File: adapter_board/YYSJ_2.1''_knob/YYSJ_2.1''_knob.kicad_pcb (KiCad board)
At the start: 2 copper layers, 80 x 80 mm, 12 parts, among them J1 USB_C_Receptacle_USB2.0, J2 FPC 10, J3 Conn_01x10

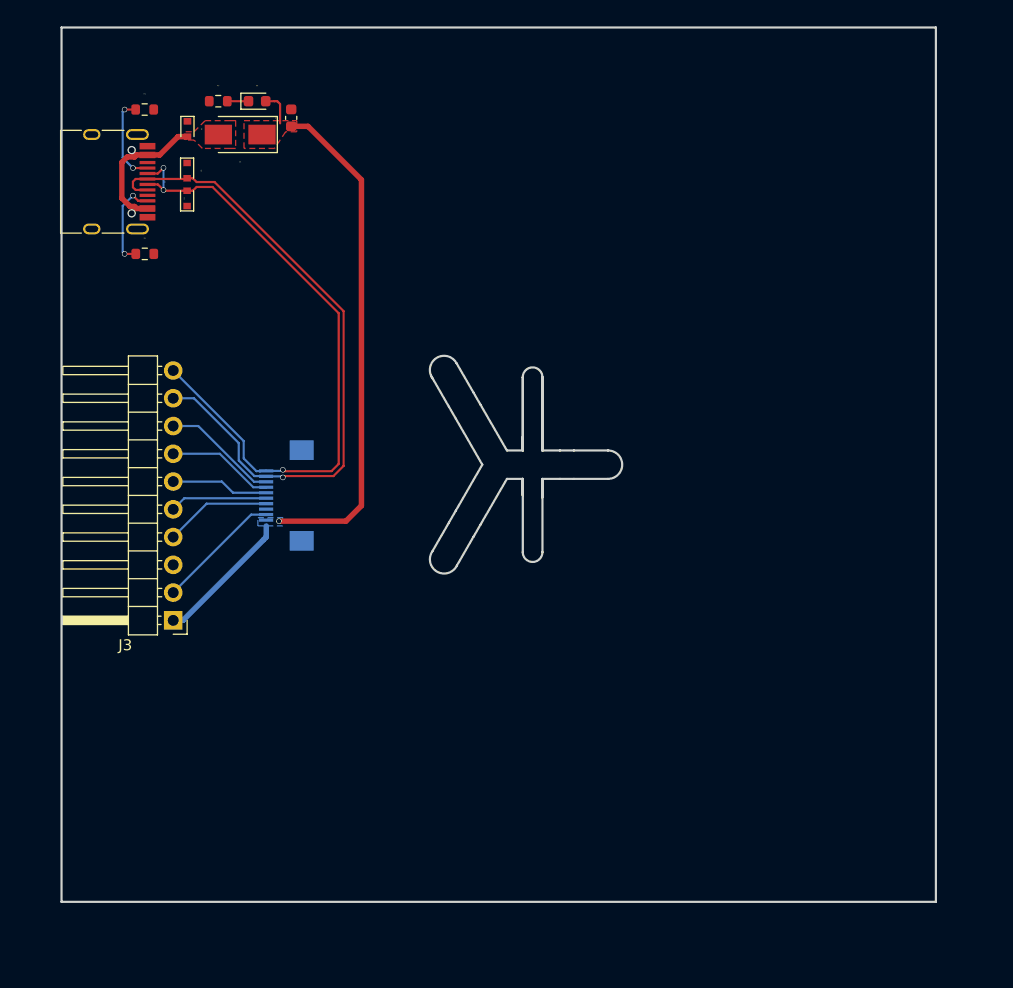
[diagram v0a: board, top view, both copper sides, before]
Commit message: adapter_board.YYSJ_2.1''knob: finish
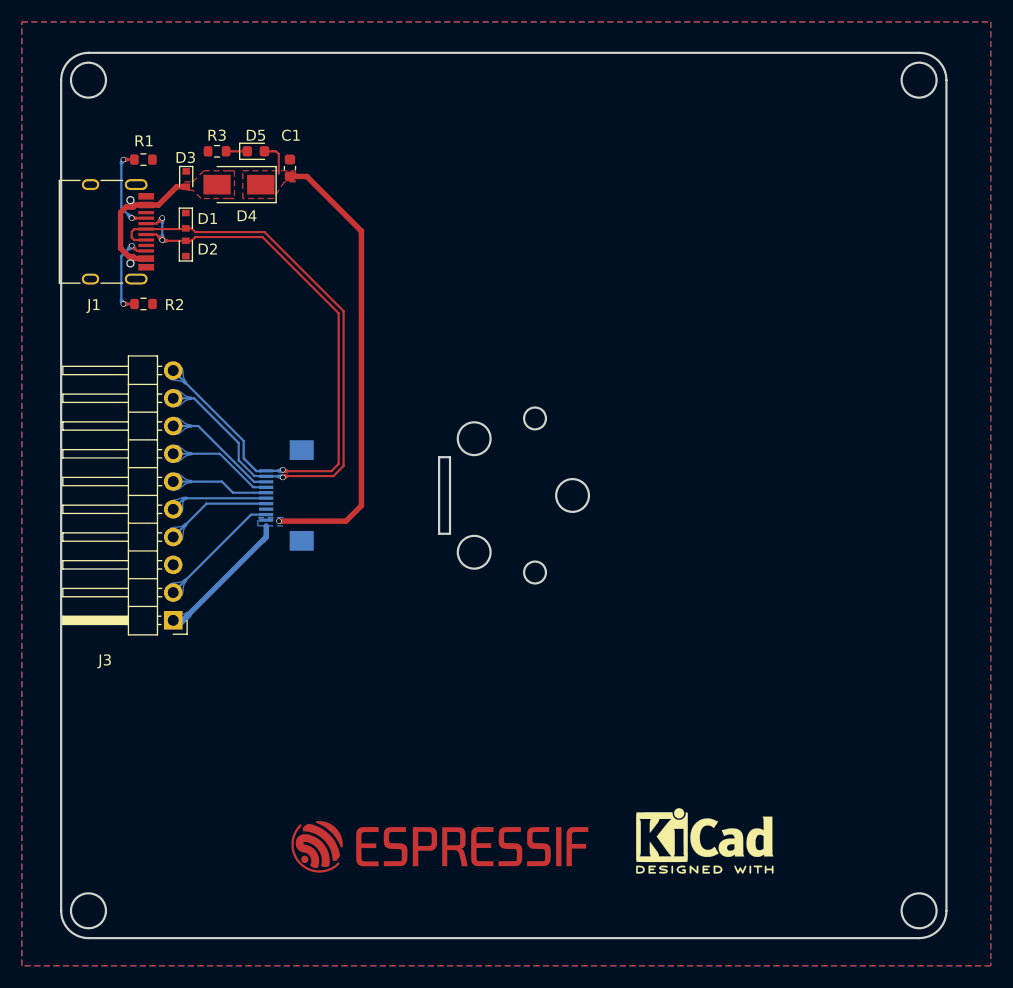
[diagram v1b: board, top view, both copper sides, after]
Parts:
- added G***: ESP_LOGO, LOGO:LOGO, F.Cu at (84.9, 161.6)
- added REF**: KiCad-Logo2_5mm_SilkScreen, Symbol:KiCad-Logo2_5mm_SilkScreen, F.Cu at (109.3, 161.1)
- moved D1 4.58 mm to (61.8, 104.4)
- moved D3 4.58 mm to (61.8, 100.6)
- moved C1 4.58 mm to (71.3, 99.6)
- moved D2 4.58 mm to (61.8, 106.9)
- moved D4 4.58 mm to (66.6, 101.1)
- moved D5 4.58 mm to (68.2, 98.0)
- moved R1 4.58 mm to (57.9, 98.8)
- moved R2 4.58 mm to (57.9, 112.0)
- moved R3 4.58 mm to (64.6, 98.0)
- moved J1 4.58 mm to (54.1, 105.4)
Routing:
- net /VCC5V: track 62.3 -> 57.7 mm
- net /USB_D-: track 60.4 -> 58.6 mm
- net /USB_D+: track 60.4 -> 58.6 mm
- added copper zone on B.Cu, net GND
- added copper zone on F.Cu, net GND
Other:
- board size 80 x 80 mm -> 81 x 81 mm
